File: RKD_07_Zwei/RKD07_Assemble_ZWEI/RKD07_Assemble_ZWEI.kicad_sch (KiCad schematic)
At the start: 179 parts, among them J1 Conn_01x24, J2 Conn_01x24, J21 Conn_01x02_Socket, J22 Conn_01x02_Socket, J23 Conn_01x10, J24 Conn_01x06, J3 Conn_01x12, J4 Conn_01x06, J51 RJ12, J52 RJ12, J53 Qwiic_RA, J6 Conn_01x06, J7 Conn_01x06, J8 Conn_01x12, SW1 SW_Push, SW10 SW_Push, SW11 SW_Push, SW12 SW_Push, SW13 SW_Push, SW14 SW_Push, SW15 SW_Push, SW16 SW_Push, SW17 SW_Push, SW18 SW_Push, SW19 SW_Push, SW2 SW_Push, SW20 SW_Push, SW21 SW_Push, SW22 SW_Push, SW23 SW_Push, SW24 SW_Push, SW25 SW_Push, SW26 SW_Push, SW27 SW_Push, SW28 SW_Push, SW29 SW_Push, SW3 SW_Push, SW30 RotaryEncoder_Switch, SW31 SW_Push, SW32 SW_Push, SW4 SW_Push, SW49 RotaryEncoder_Switch, SW5 SW_Push, SW50 SW_Push, SW51 SW_Push, SW52 SW_Push, SW53 SW_Push, SW54 SW_Push, SW55 SW_Push, SW56 SW_Push, SW57 SW_Push, SW58 SW_Push, SW59 SW_Push, SW6 SW_Push, SW60 SW_Push, SW61 SW_Push, SW62 SW_Push, SW63 SW_Push, SW64 SW_Push, SW65 SW_Push, SW66 SW_Push, SW67 SW_Push, SW68 SW_Push, SW69 SW_Push, SW7 SW_Push, SW70 SW_Push, SW71 SW_Push, SW72 SW_Push, SW73 SW_Push, SW74 SW_Push, SW75 SW_Push, SW76 SW_Push, SW77 SW_Push, SW78 SW_Push, SW79 SW_Push, SW8 SW_Push, SW80 SW_Push, SW81 SW_Push, SW82 SW_Push, SW83 SW_Push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

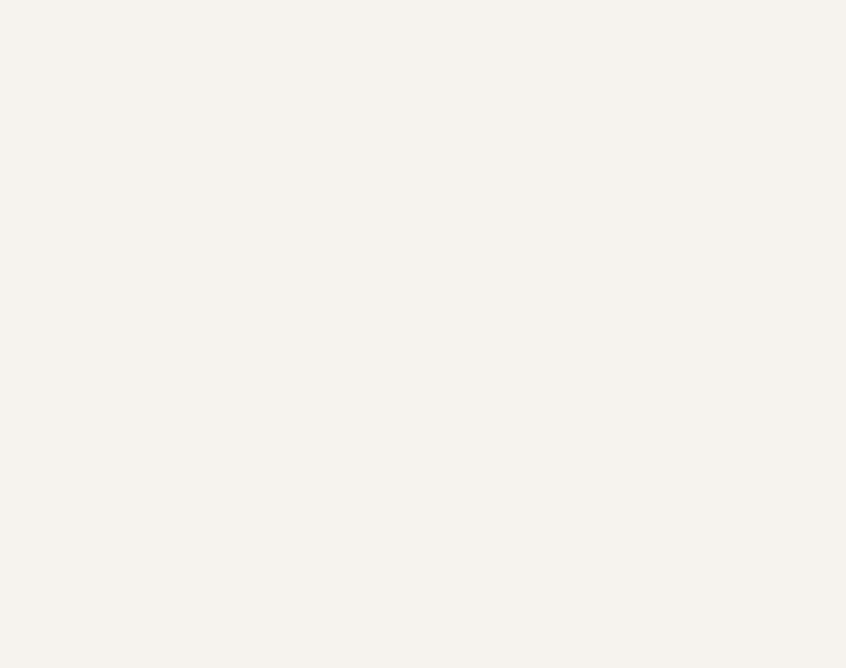
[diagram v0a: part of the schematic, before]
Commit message: update
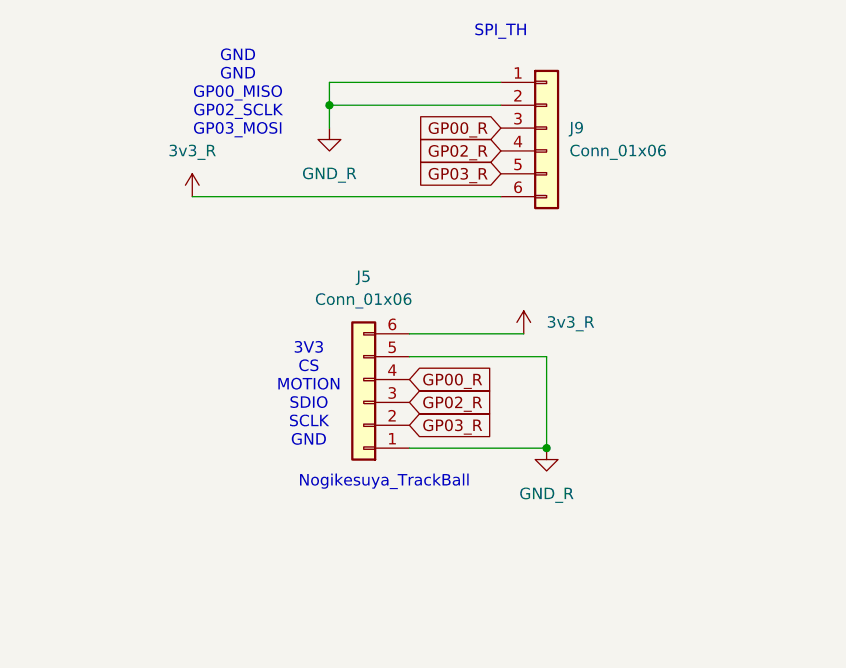
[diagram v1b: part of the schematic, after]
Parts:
- added J5: Conn_01x06, Connector_FFC-FPC:Hirose_FH12-6S-0.5SH_1x06-1MP_P0.50mm_Horizontal, symbol Connector_Generic:Conn_01x06
- added J9: Conn_01x06, Connector_PinHeader_2.54mm:PinHeader_1x06_P2.54mm_Vertical, symbol Connector_Generic:Conn_01x06
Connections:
- net 3v3_R: now also J5.6 (Pin_6), J9.6 (Pin_6)
- net GND_R: now also J5.1 (Pin_1), J5.5 (Pin_5), J9.1 (Pin_1), J9.2 (Pin_2)
- net GP00_R: now also J5.4 (Pin_4), J9.3 (Pin_3)
- net GP02_R: now also J5.3 (Pin_3), J9.4 (Pin_4)
- net GP03_R: now also J5.2 (Pin_2), J9.5 (Pin_5)
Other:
- note added: "GND GND GP00_MISO GP02_SCLK GP03_MOSI"
- note added: "Nogikesuya_TrackBall"
- note added: "SPI_TH"
